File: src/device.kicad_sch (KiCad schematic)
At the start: 0 parts

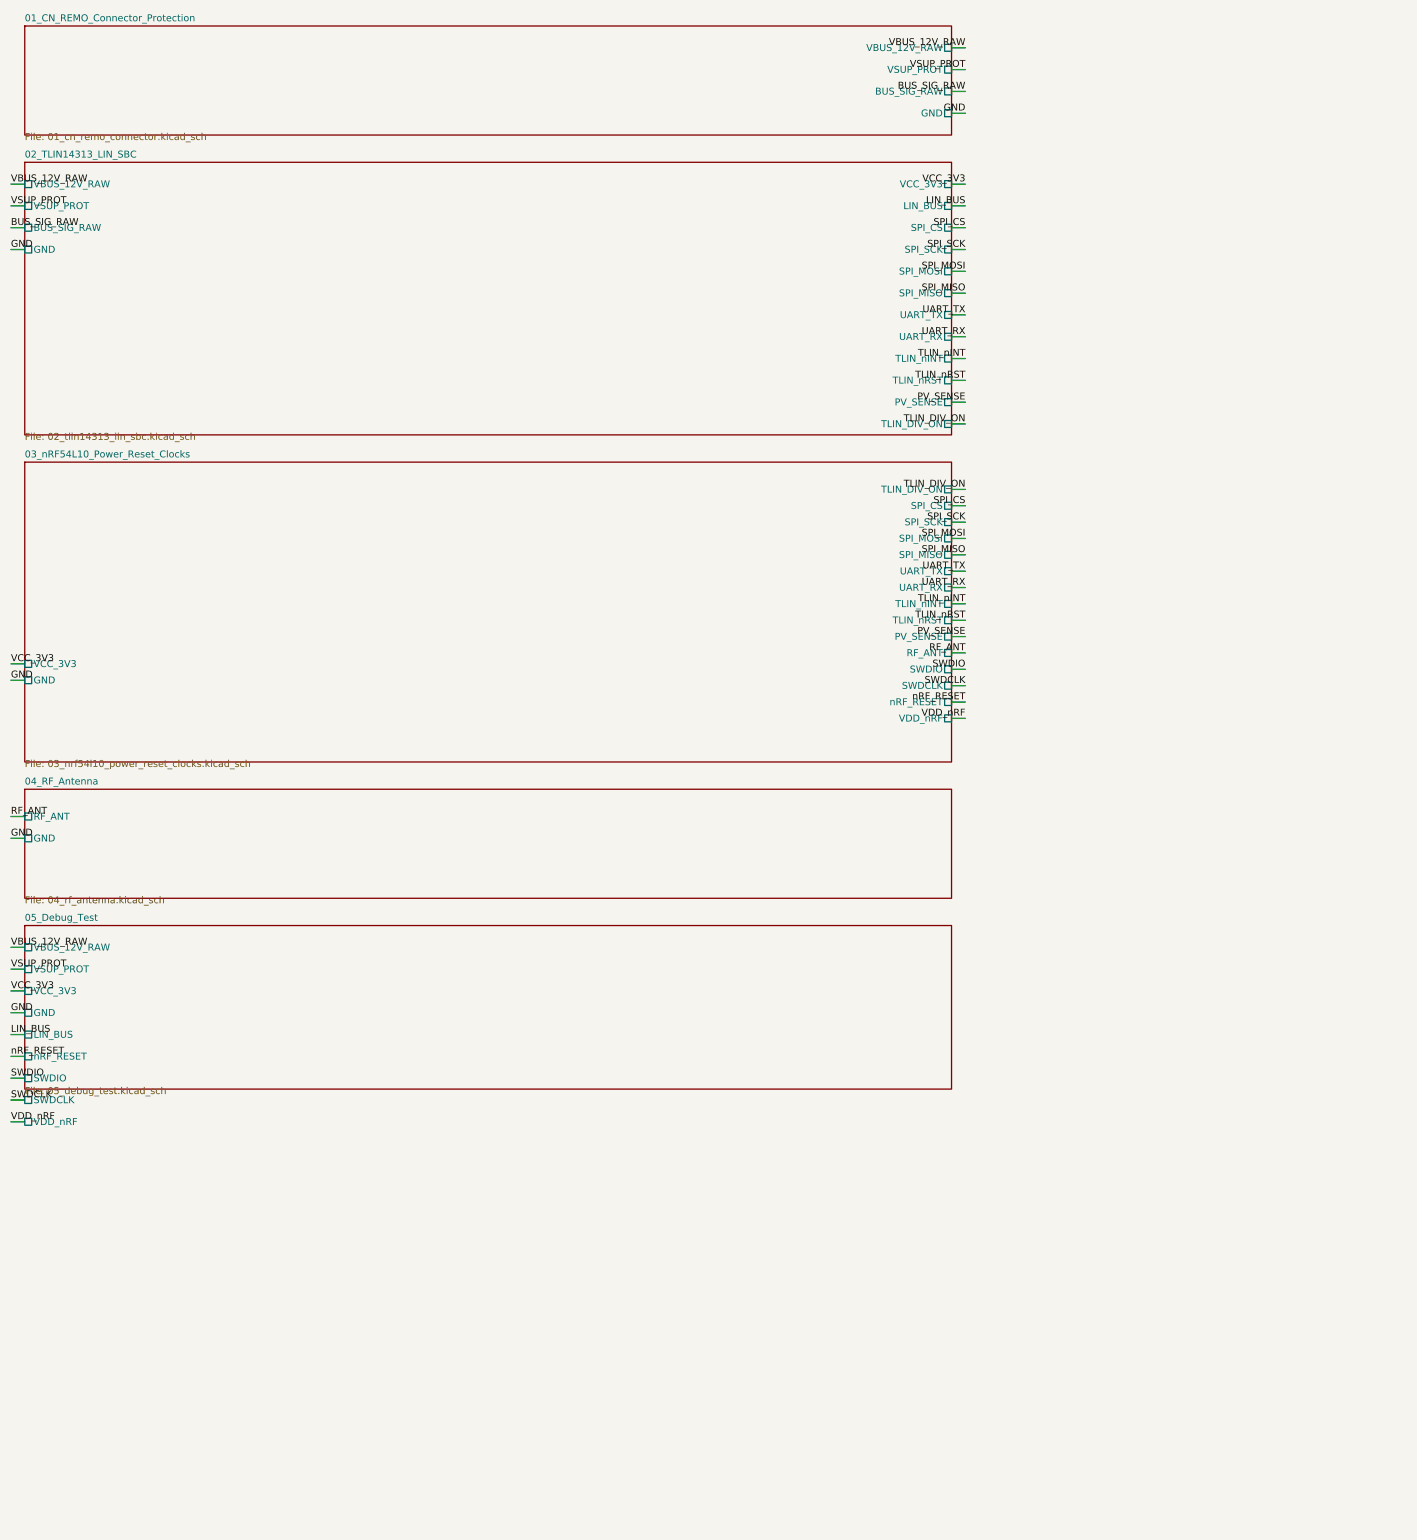
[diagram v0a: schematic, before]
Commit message: stage
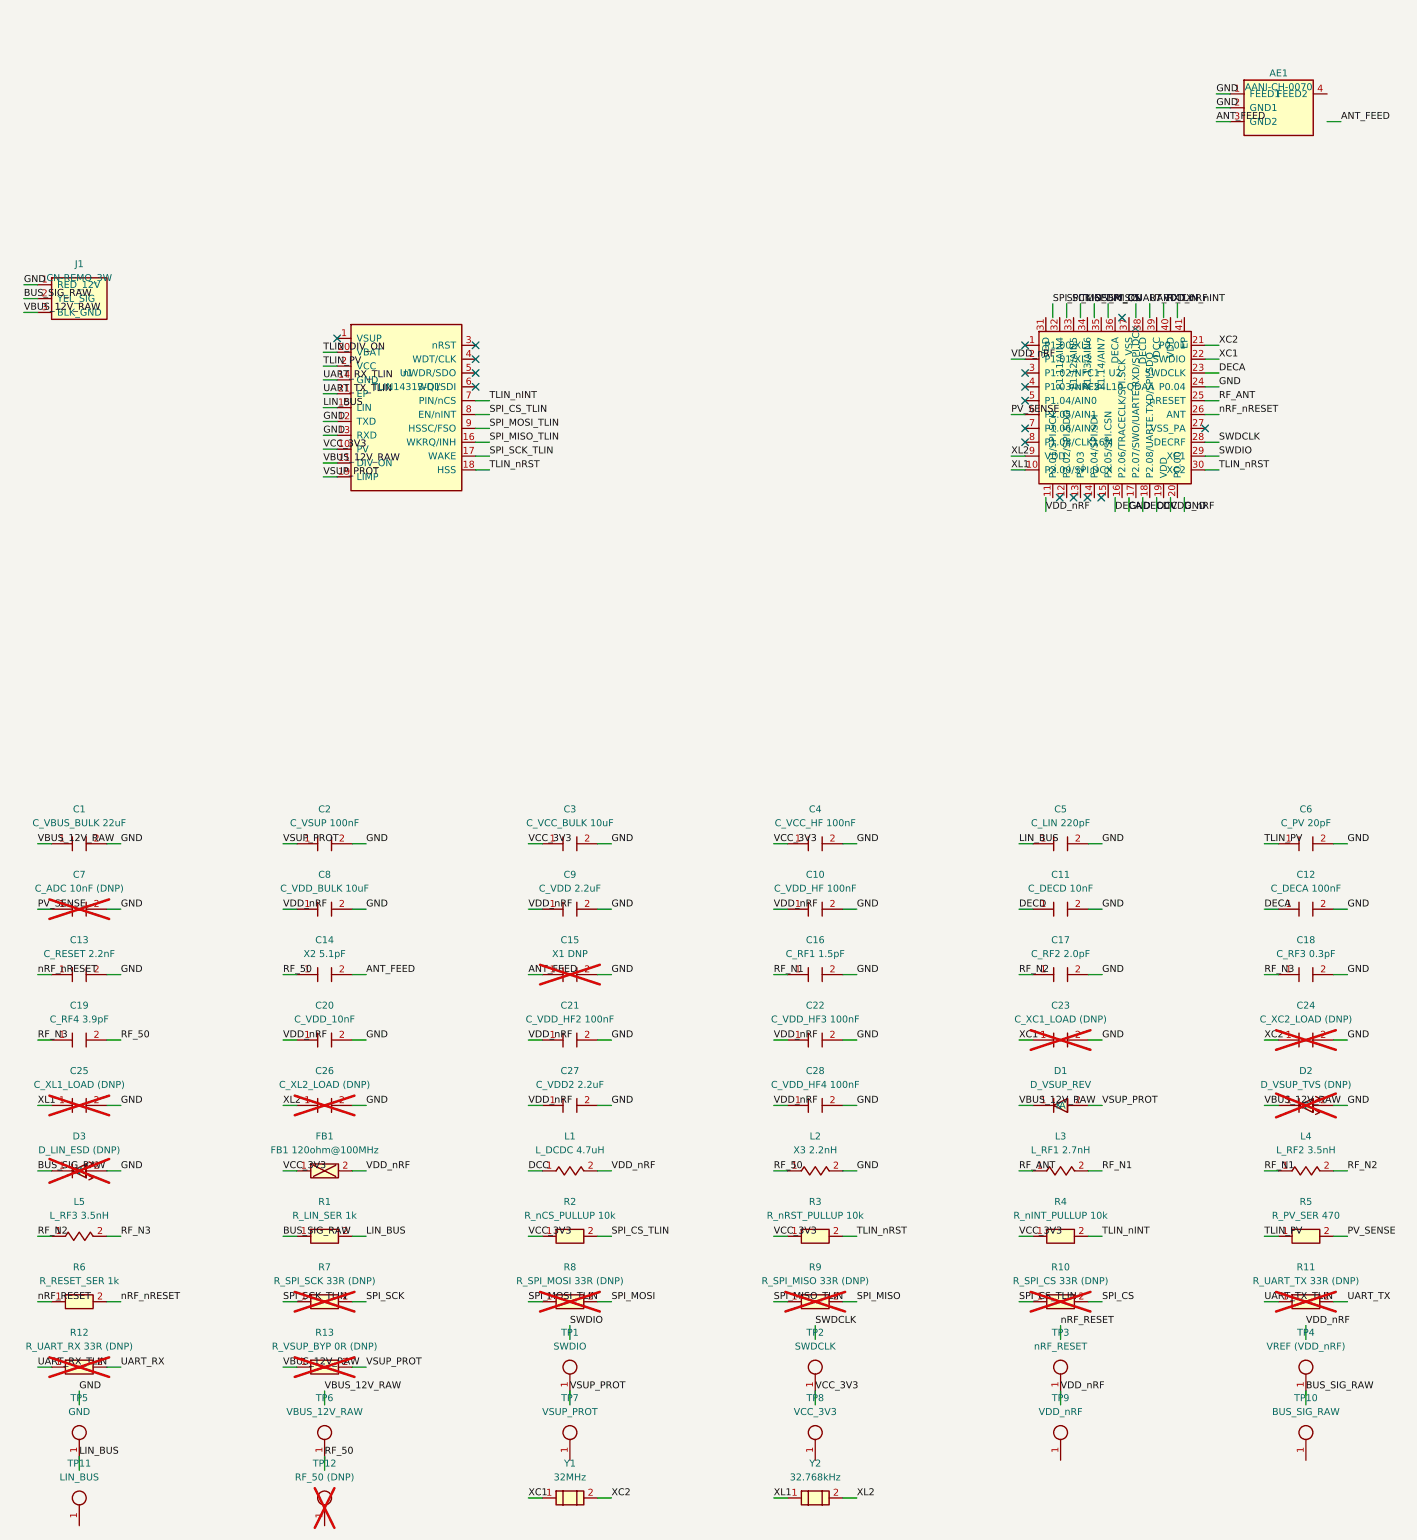
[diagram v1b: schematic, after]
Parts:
- added AE1: AANI-CH-0070, RF_Antenna:Abracon_AANI-CH-0070, symbol Device:AANI-CH-0070
- added C1: C_VBUS_BULK 22uF, Capacitor_SMD:C_0805_2012Metric, symbol Device:C
- added C10: C_VDD_HF 100nF, Capacitor_SMD:C_0402_1005Metric, symbol Device:C
- added C11: C_DECD 10nF, Capacitor_SMD:C_0402_1005Metric, symbol Device:C
- added C12: C_DECA 100nF, Capacitor_SMD:C_0402_1005Metric, symbol Device:C
- added C13: C_RESET 2.2nF, Capacitor_SMD:C_0402_1005Metric, symbol Device:C
- added C14: X2 5.1pF, Capacitor_SMD:C_0402_1005Metric, symbol Device:C
- added C15: X1 DNP, Capacitor_SMD:C_0402_1005Metric, symbol Device:C
- added C16: C_RF1 1.5pF, Capacitor_SMD:C_0402_1005Metric, symbol Device:C
- added C17: C_RF2 2.0pF, Capacitor_SMD:C_0402_1005Metric, symbol Device:C
- added C18: C_RF3 0.3pF, Capacitor_SMD:C_0402_1005Metric, symbol Device:C
- added C19: C_RF4 3.9pF, Capacitor_SMD:C_0402_1005Metric, symbol Device:C
- added C2: C_VSUP 100nF, Capacitor_SMD:C_0402_1005Metric, symbol Device:C
- added C20: C_VDD_10nF, Capacitor_SMD:C_0402_1005Metric, symbol Device:C
- added C21: C_VDD_HF2 100nF, Capacitor_SMD:C_0402_1005Metric, symbol Device:C
- added C22: C_VDD_HF3 100nF, Capacitor_SMD:C_0402_1005Metric, symbol Device:C
- added C23: C_XC1_LOAD (DNP), Capacitor_SMD:C_0402_1005Metric, symbol Device:C
- added C24: C_XC2_LOAD (DNP), Capacitor_SMD:C_0402_1005Metric, symbol Device:C
- added C25: C_XL1_LOAD (DNP), Capacitor_SMD:C_0402_1005Metric, symbol Device:C
- added C26: C_XL2_LOAD (DNP), Capacitor_SMD:C_0402_1005Metric, symbol Device:C
- added C27: C_VDD2 2.2uF, Capacitor_SMD:C_0402_1005Metric, symbol Device:C
- added C28: C_VDD_HF4 100nF, Capacitor_SMD:C_0402_1005Metric, symbol Device:C
- added C3: C_VCC_BULK 10uF, Capacitor_SMD:C_0603_1608Metric, symbol Device:C
- added C4: C_VCC_HF 100nF, Capacitor_SMD:C_0402_1005Metric, symbol Device:C
- added C5: C_LIN 220pF, Capacitor_SMD:C_0402_1005Metric, symbol Device:C
- added C6: C_PV 20pF, Capacitor_SMD:C_0402_1005Metric, symbol Device:C
- added C7: C_ADC 10nF (DNP), Capacitor_SMD:C_0402_1005Metric, symbol Device:C
- added C8: C_VDD_BULK 10uF, Capacitor_SMD:C_0603_1608Metric, symbol Device:C
- added C9: C_VDD 2.2uF, Capacitor_SMD:C_0402_1005Metric, symbol Device:C
- added D1: D_VSUP_REV, Diode_SMD:D_SMA, symbol Device:D_Schottky
- added D2: D_VSUP_TVS (DNP), Diode_SMD:D_SMB, symbol Device:D_TVS
- added D3: D_LIN_ESD (DNP), Diode_SMD:D_SOD-523, symbol Device:D_TVS
- added FB1: FB1 120ohm@100MHz, Ferrite_Bead_SMD:Ferrite_Bead_0603_1608Metric, symbol Device:Ferrite_Bead
- added J1: CN-REMO_3W, symbol Device:CN-REMO_3W
- added L1: L_DCDC 4.7uH, Inductor_SMD:L_0603_1608Metric, symbol Device:L
- added L2: X3 2.2nH, Inductor_SMD:L_0402_1005Metric, symbol Device:L
- added L3: L_RF1 2.7nH, Inductor_SMD:L_0402_1005Metric, symbol Device:L
- added L4: L_RF2 3.5nH, Inductor_SMD:L_0402_1005Metric, symbol Device:L
- added L5: L_RF3 3.5nH, Inductor_SMD:L_0402_1005Metric, symbol Device:L
- added R1: R_LIN_SER 1k, Resistor_SMD:R_0402_1005Metric, symbol Device:R
- added R10: R_SPI_CS 33R (DNP), Resistor_SMD:R_0402_1005Metric, symbol Device:R
- added R11: R_UART_TX 33R (DNP), Resistor_SMD:R_0402_1005Metric, symbol Device:R
- added R12: R_UART_RX 33R (DNP), Resistor_SMD:R_0402_1005Metric, symbol Device:R
- added R13: R_VSUP_BYP 0R (DNP), Resistor_SMD:R_0603_1608Metric, symbol Device:R
- added R2: R_nCS_PULLUP 10k, Resistor_SMD:R_0402_1005Metric, symbol Device:R
- added R3: R_nRST_PULLUP 10k, Resistor_SMD:R_0402_1005Metric, symbol Device:R
- added R4: R_nINT_PULLUP 10k, Resistor_SMD:R_0402_1005Metric, symbol Device:R
- added R5: R_PV_SER 470, Resistor_SMD:R_0402_1005Metric, symbol Device:R
- added R6: R_RESET_SER 1k, Resistor_SMD:R_0402_1005Metric, symbol Device:R
- added R7: R_SPI_SCK 33R (DNP), Resistor_SMD:R_0402_1005Metric, symbol Device:R
- added R8: R_SPI_MOSI 33R (DNP), Resistor_SMD:R_0402_1005Metric, symbol Device:R
- added R9: R_SPI_MISO 33R (DNP), Resistor_SMD:R_0402_1005Metric, symbol Device:R
- added TP1: SWDIO, TestPoint:TestPoint_Pad_D1.0mm, symbol Device:TestPoint
- added TP10: BUS_SIG_RAW, TestPoint:TestPoint_Pad_D1.0mm, symbol Device:TestPoint
- added TP11: LIN_BUS, TestPoint:TestPoint_Pad_D1.0mm, symbol Device:TestPoint
- added TP12: RF_50 (DNP), TestPoint:TestPoint_Pad_D1.0mm, symbol Device:TestPoint
- added TP2: SWDCLK, TestPoint:TestPoint_Pad_D1.0mm, symbol Device:TestPoint
- added TP3: nRF_RESET, TestPoint:TestPoint_Pad_D1.0mm, symbol Device:TestPoint
- added TP4: VREF (VDD_nRF), TestPoint:TestPoint_Pad_D1.0mm, symbol Device:TestPoint
- added TP5: GND, TestPoint:TestPoint_Pad_D1.0mm, symbol Device:TestPoint
- added TP6: VBUS_12V_RAW, TestPoint:TestPoint_Pad_D1.0mm, symbol Device:TestPoint
- added TP7: VSUP_PROT, TestPoint:TestPoint_Pad_D1.0mm, symbol Device:TestPoint
- added TP8: VCC_3V3, TestPoint:TestPoint_Pad_D1.0mm, symbol Device:TestPoint
- added TP9: VDD_nRF, TestPoint:TestPoint_Pad_D1.0mm, symbol Device:TestPoint
- added U1: TLIN14313-Q1, Package_DFN_QFN:VQFN-20-1EP_4.5x3.5mm_P0.5mm, symbol Device:TLIN14313-Q1
- added U2: nRF54L10-QDAA, Package_DFN_QFN:QFN-40-1EP_5x5mm_P0.4mm, symbol Device:nRF54L10-QDAA
- added Y1: 32MHz, Crystal:Crystal_SMD_2016-2Pin_2.0x1.6mm, symbol Device:Crystal
- added Y2: 32.768kHz, Crystal:Crystal_SMD_2012-2Pin_2.0x1.2mm, symbol Device:Crystal
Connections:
- net BUS_SIG_RAW: now also D3.1 (A), J1.2 (YEL_SIG), R1.1
- net GND: now also AE1.1 (FEED1), AE1.2 (GND1), C1.2, C10.2, C11.2, C12.2, C13.2, C15.2, C16.2, C17.2, C18.2, C2.2, C20.2, C21.2, C22.2, C23.2, C24.2, C25.2, C26.2, C27.2, C28.2, C3.2, C4.2, C5.2, C6.2, C7.2, C8.2, C9.2, D2.2 (K), D3.2 (K), J1.1 (RED_12V), L2.2, U1.12 (TXD), U1.13 (RXD), U2.24 (P0.04)
- net LIN_BUS: now also C5.1, R1.2, U1.15 (LIN)
- net PV_SENSE: now also C7.1, R5.2, U2.6 (P1.05/AIN1)
- net RF_ANT: now also L3.1, U2.25 (nRESET)
- net SPI_CS: now also R10.2
- net SPI_MISO: now also R9.2
- net SPI_MOSI: now also R8.2
- net SPI_SCK: now also R7.2
- net SWDCLK: now also U2.28 (DECRF)
- net SWDIO: now also U2.29 (XC1)
- net TLIN_DIV_ON: now also U1.20 (VBAT)
- net TLIN_nINT: now also R4.2, U1.7 (PIN/nCS)
- net TLIN_nRST: now also R3.2, U1.18 (HSS), U2.30 (XC2)
- net UART_RX: now also R12.2
- net UART_TX: now also R11.2
- net VBUS_12V_RAW: now also C1.1, D1.1 (A), D2.1 (A), J1.3 (BLK_GND), R13.1, U1.11 (DIV_ON)
- net VCC_3V3: now also C3.1, C4.1, FB1.1, R2.1, R3.1, R4.1, U1.10 (PV)
- net VDD_nRF: now also C10.1, C20.1, C21.1, C22.1, C27.1, C28.1, C8.1, C9.1, FB1.2, L1.2, U2.2 (P1.01/XL2)
- net VSUP_PROT: now also C2.1, D1.2 (K), R13.2, U1.19 (LIMP)
- net nRF_RESET: now also R6.1
- new net ANT_FEED: AE1.3 (GND2), C14.2, C15.1
- new net DCC: L1.1
- new net DECA: C12.1, U2.23 (SWDCLK)
- new net DECD: C11.1
- new net RF_50: C14.1, C19.2, L2.1
- new net RF_N1: C16.1, L3.2, L4.1
- new net RF_N2: C17.1, L4.2, L5.1
- new net RF_N3: C18.1, C19.1, L5.2
- new net SPI_CS_TLIN: R10.1, R2.2, U1.8 (EN/nINT)
- new net SPI_MISO_TLIN: R9.1, U1.16 (WKRQ/INH)
- new net SPI_MOSI_TLIN: R8.1, U1.9 (HSSC/FSO)
- new net SPI_SCK_TLIN: R7.1, U1.17 (WAKE)
- new net TLIN_PV: C6.1, R5.1, U1.2 (VCC)
- new net UART_RX_TLIN: R12.1, U1.14 (GND)
- new net UART_TX_TLIN: R11.1, U1.21 (EP)
- new net XC1: C23.1, U2.22 (SWDIO), Y1.1
- new net XC2: C24.1, U2.21 (P0.01), Y1.2
- new net XL1: C25.1, U2.10 (P2.00/SPI.DCX), Y2.1
- new net XL2: C26.1, U2.9 (VDD), Y2.2
- new net nRF_nRESET: C13.1, R6.2, U2.26 (ANT)
- no-connect marks 0 -> 17
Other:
- removed sheet 01_CN_REMO_Connector_Protection
- removed sheet 02_TLIN14313_LIN_SBC
- removed sheet 03_nRF54L10_Power_Reset_Clocks
- removed sheet 04_RF_Antenna
- removed sheet 05_Debug_Test
- title: (none) -> PREMTA Slave Controller

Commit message: stage
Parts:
- AE1: symbol Device:AANI-CH-0070 -> device:AANI-CH-0070
- C1, C10, C11, C12, C13, C14, C15, C16, C17, C18, C19, C2, C20, C21, C22, C23, C24, C25, C26, C27, C28, C3, C4, C5, C6, C7, C8, C9: symbol Device:C -> device:C
- D1: symbol Device:D_Schottky -> device:D_Schottky
- D2, D3: symbol Device:D_TVS -> device:D_TVS
- FB1: symbol Device:Ferrite_Bead -> device:Ferrite_Bead
- J1: symbol Device:CN-REMO_3W -> device:CN-REMO_3W
- L1, L2, L3, L4, L5: symbol Device:L -> device:L
- R1, R10, R11, R12, R13, R2, R3, R4, R5, R6, R7, R8, R9: symbol Device:R -> device:R
- TP1, TP10, TP11, TP12, TP2, TP3, TP4, TP5, TP6, TP7, TP8, TP9: symbol Device:TestPoint -> device:TestPoint
- U1: symbol Device:TLIN14313-Q1 -> device:TLIN14313-Q1
- U2: symbol Device:nRF54L10-QDAA -> device:nRF54L10-QDAA
- Y1, Y2: symbol Device:Crystal -> device:Crystal
